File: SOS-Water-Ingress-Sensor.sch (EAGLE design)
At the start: 12 parts

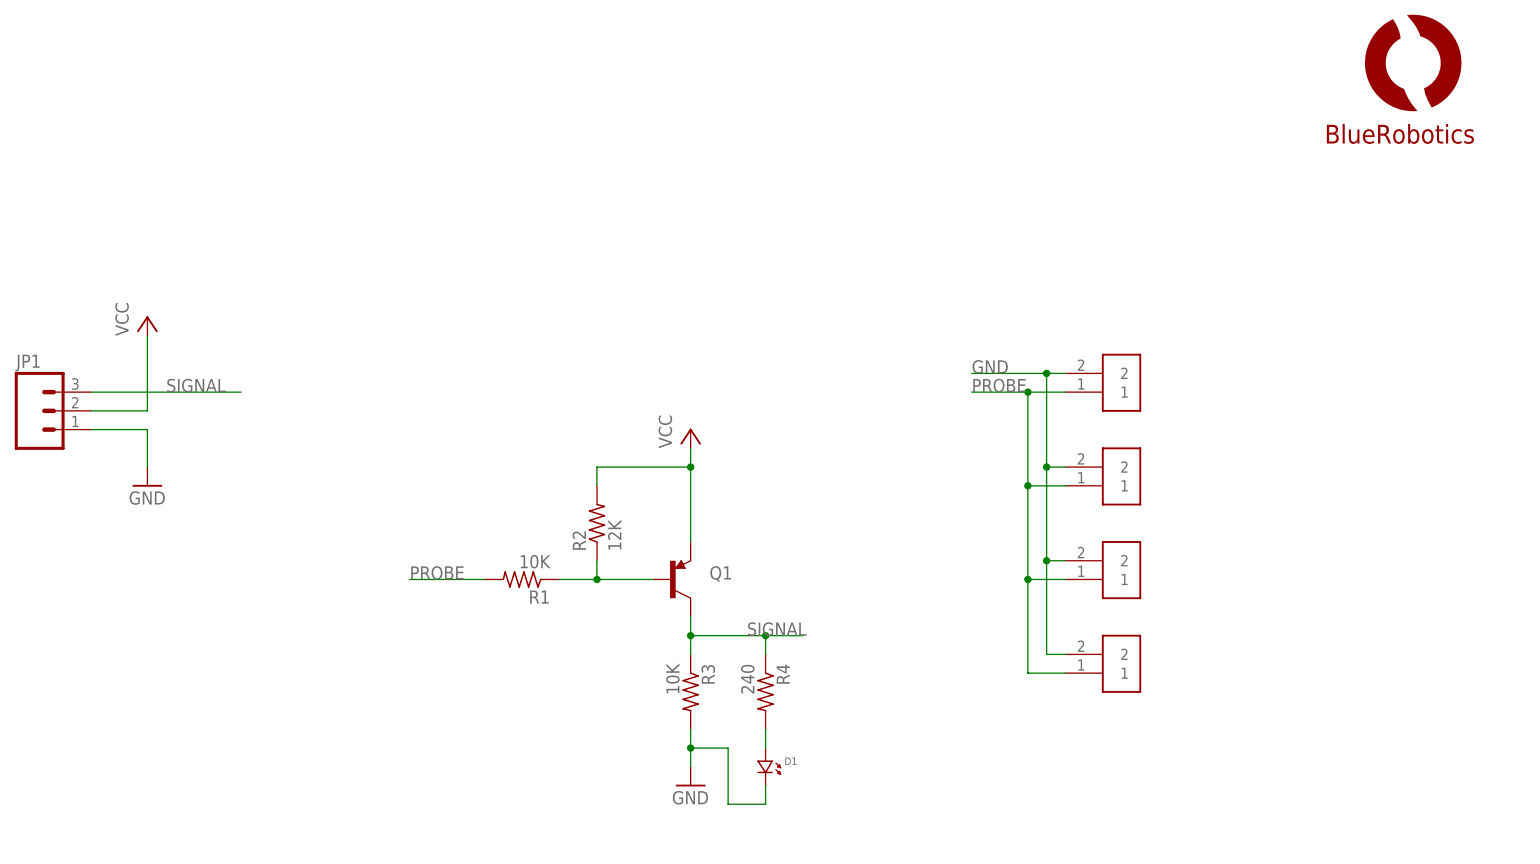
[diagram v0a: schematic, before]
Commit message: Minor tweaks to layout all around.
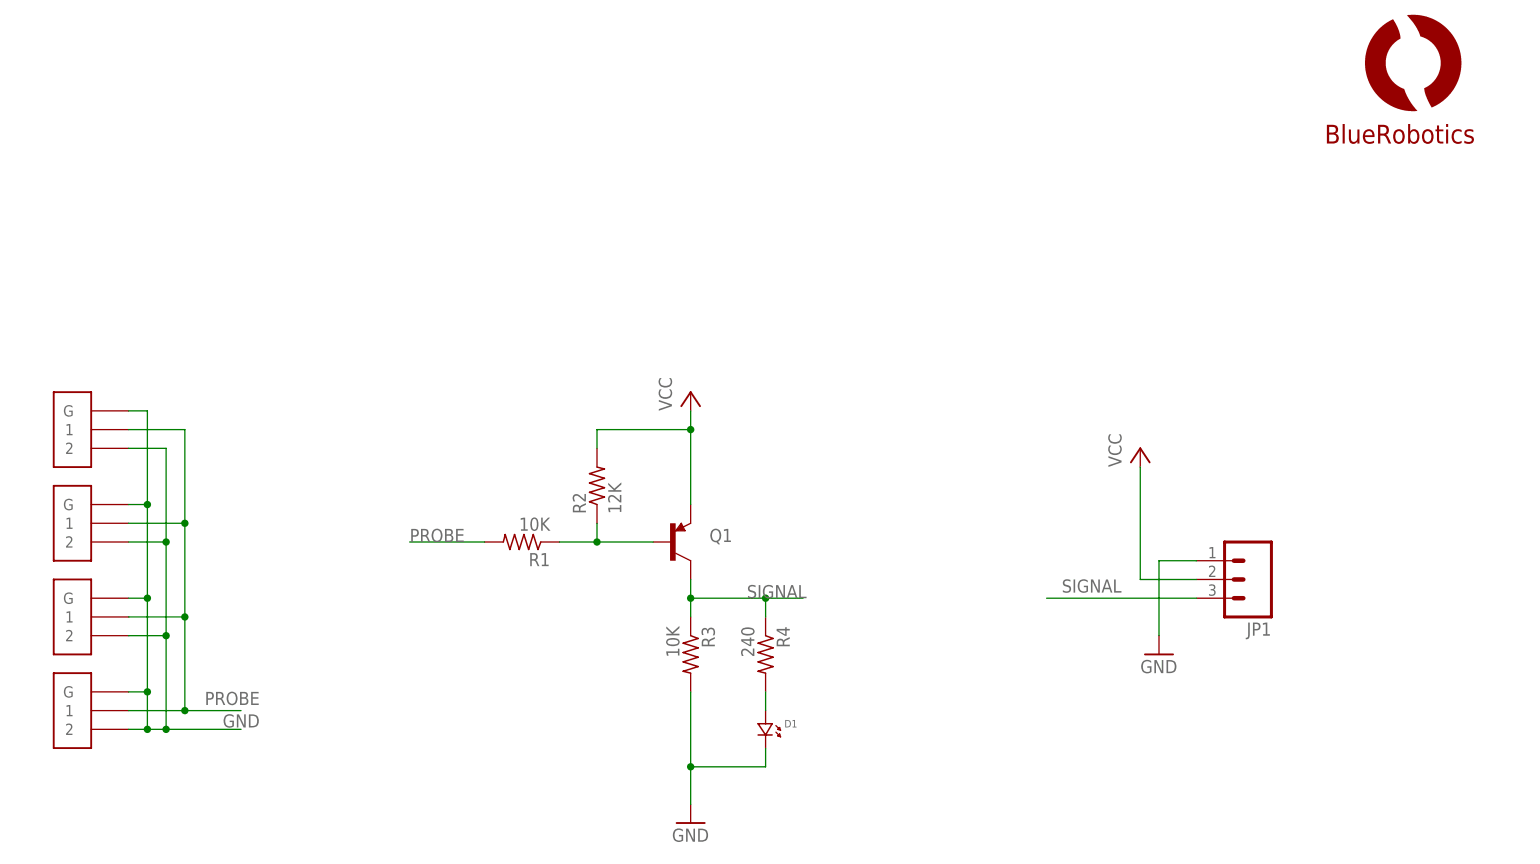
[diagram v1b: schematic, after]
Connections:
- net GND: now also U$1.G, U$2.G, U$3.G, U$4.G
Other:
- moved on the sheet: D1, JP1, Q1, R1, R2, R3, R4
